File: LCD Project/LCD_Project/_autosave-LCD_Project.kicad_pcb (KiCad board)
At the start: 2 copper layers, 109 x 88.5 mm, 6 parts, among them J1 DT15-4P, U1 Teensy4.0, U2 MIC5365-1.3YC5-TR

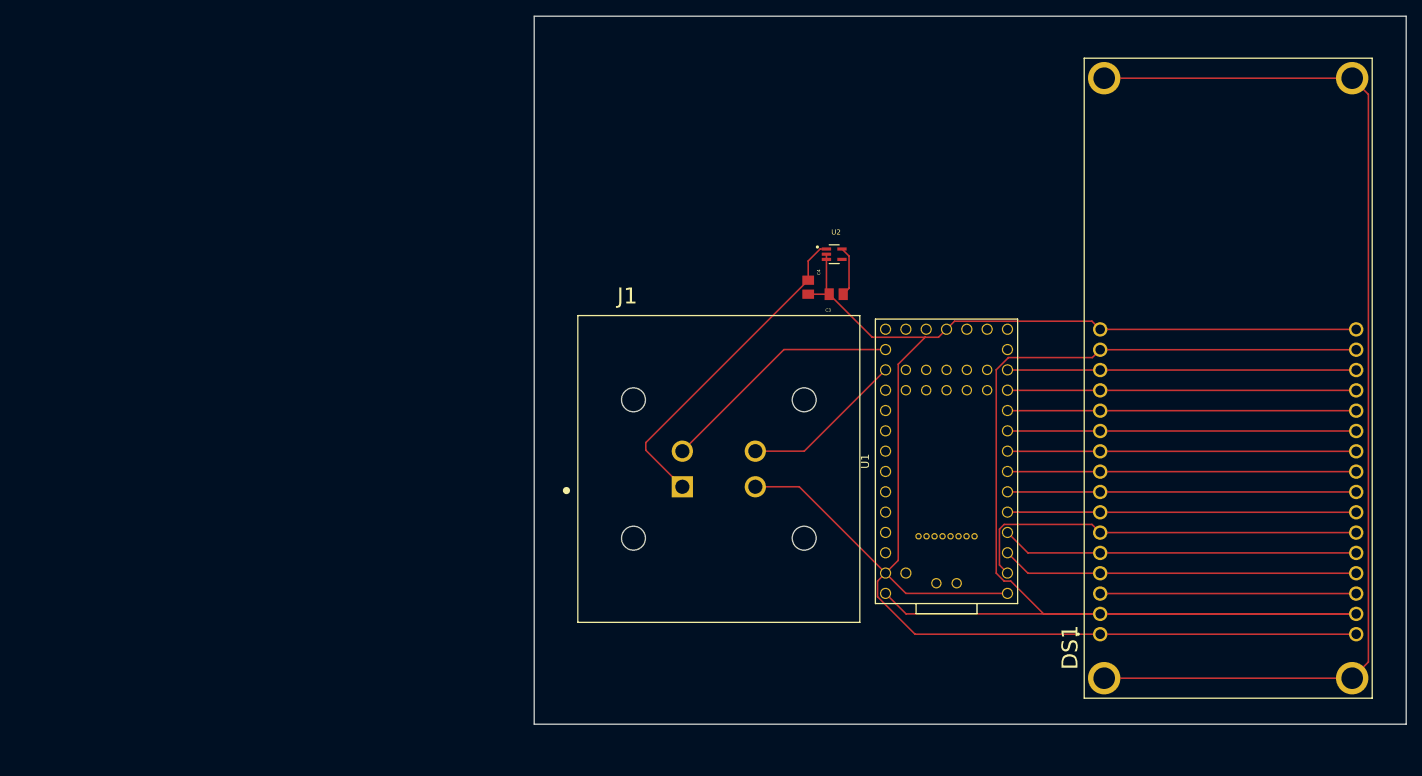
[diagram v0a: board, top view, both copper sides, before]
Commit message: Add files via upload
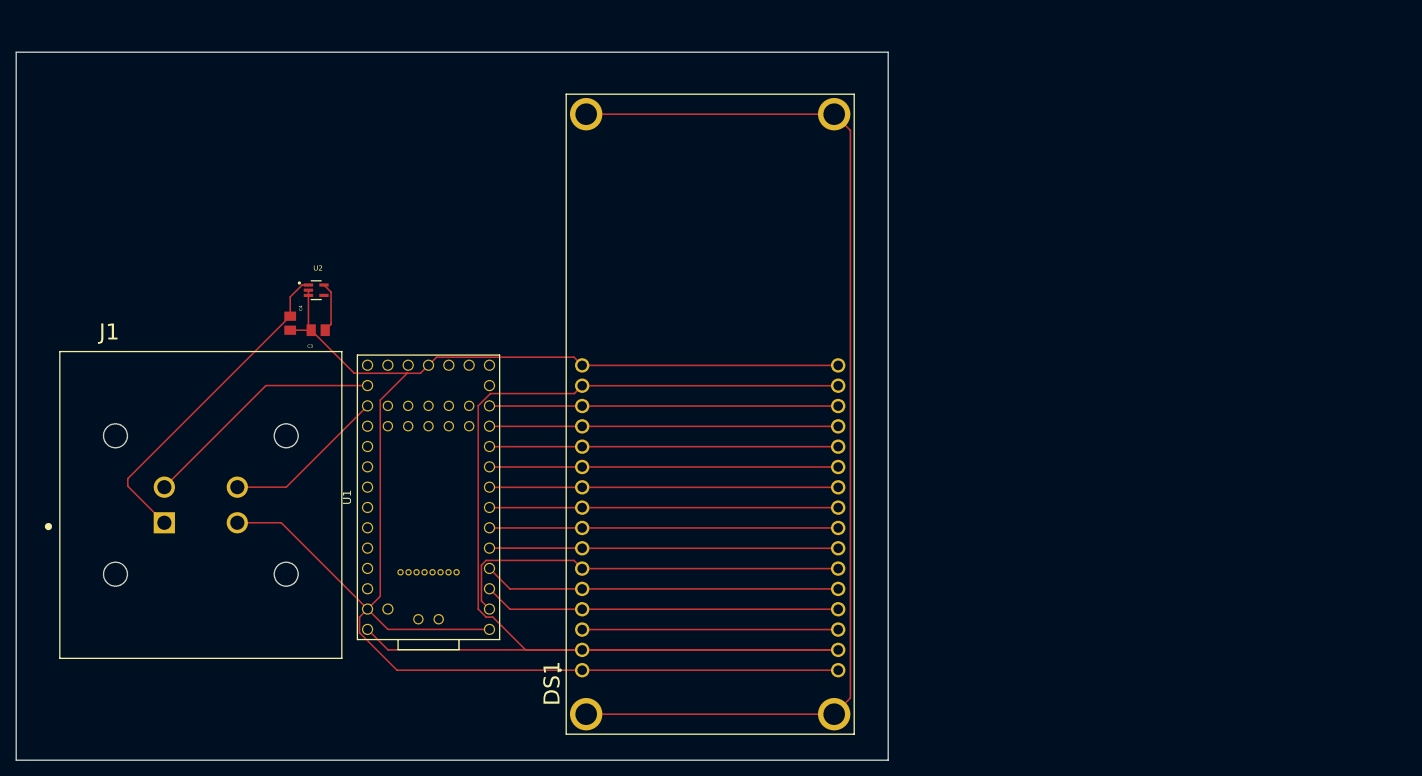
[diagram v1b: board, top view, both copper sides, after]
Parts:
- moved J1 64.9 mm to (103.3, 105.6)
- moved C3 64.9 mm to (118.0, 83.8)
- moved C4 64.9 mm to (114.5, 82.9)
- moved DS1 64.9 mm to (167.0, 94.2)
- moved U1 64.9 mm to (131.8, 104.6)
- moved U2 64.9 mm to (117.8, 78.8)
